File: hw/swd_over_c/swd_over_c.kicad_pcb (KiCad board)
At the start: 4 copper layers, 18.3 x 16 mm, 17 parts, among them J1 USB_C_Receptacle_USB2.0, J2 Conn_ARM_JTAG_SWD_10, P1 USB_C_Plug, U1 ATtiny24-20M

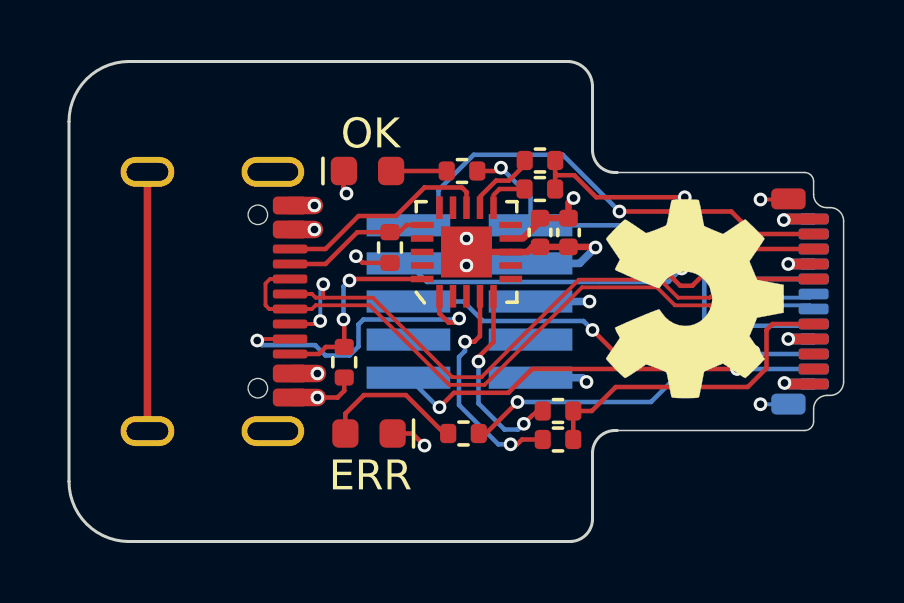
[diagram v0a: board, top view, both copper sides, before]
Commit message: SWD over USB-C v1.4!!!
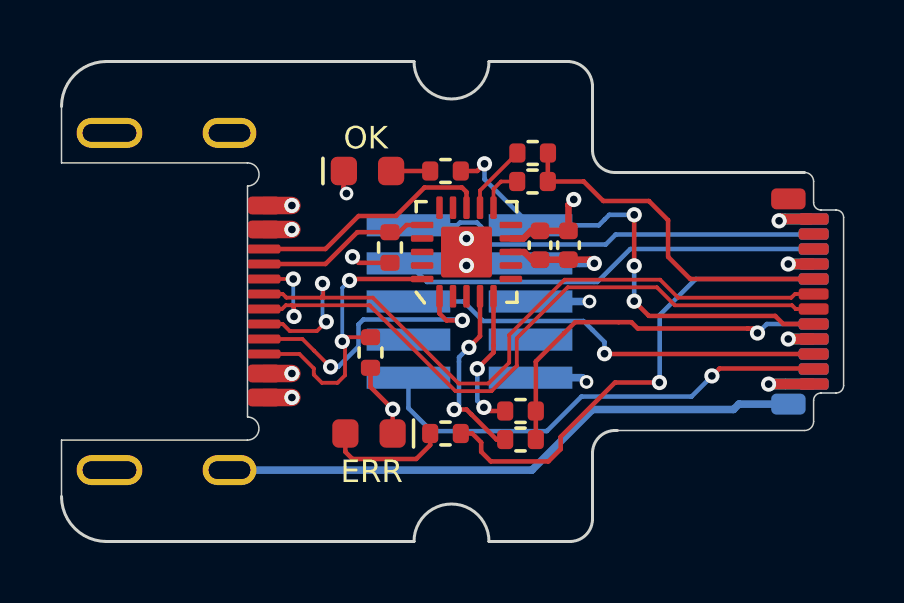
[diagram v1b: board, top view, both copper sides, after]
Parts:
- J1: value USB_C_Receptacle_USB2.0 -> USB-C Receptacle; footprint alvarop:USB4105-GF-A -> alvarop:USB4500-03
- P1: moved to F.Cu
- R3: value 10k -> 22k
- R4: value 22k -> 56k
- R5: value 22k -> 10k
- R6: value 56k -> 22k
- REF**: moved to B.Cu
- U1: footprint ultralibrarian:ATTINY24A-MMH -> ultralibrarian:ATTINY24A-MMH_MOD
- moved J1 1.42 mm to (161.2, 67.5)
- moved R5 1.25 mm to (170.3, 72.1)
- moved R6 1.25 mm to (170.3, 71.2), turned to 0 degrees
- moved R1 0.93 mm to (165.3, 69.2)
- moved R8 0.60 mm to (167.8, 71.9)
- moved R7 0.55 mm to (167.8, 63.1)
- moved C1 0.42 mm to (170.9, 65.6)
- moved C2 0.42 mm to (171.9, 65.6)
- moved R3 0.35 mm to (170.7, 63.5), turned to 180 degrees
- moved R4 0.35 mm to (170.7, 62.5), turned to 180 degrees
- moved REF** 0.15 mm to (176.1, 67.5), turned to 90 degrees
- turned P1 to -90 degrees
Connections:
- R3 pad 1: /CC1_R1 -> /CC1
- R3 pad 2: /CC1 -> /CC1_R1
- R4 pad 1: /CC1_R2 -> /CC1
- R4 pad 2: /CC1 -> /CC1_R2
- R6 pad 1: /CC2 -> /CC2_R2
- R6 pad 2: /CC2_R2 -> /CC2
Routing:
- net /SHIELD: track 57.0 -> 19.5 mm, vias 2 -> 0
- net /CC2_IN_MISO: track 6.65 -> 10.1 mm
- net /D+: track 23.2 -> 26.0 mm, vias 3 -> 2
- net /SBU2: track 14.4 -> 16.4 mm, vias 2 -> 1
- net /CC2: track 10.9 -> 12.7 mm, vias 0 -> 1
- net /CC2_R2: track 6.54 -> 4.78 mm
- net /D-: track 22.9 -> 24.5 mm, vias 1 -> 2
- net /NRST: track 14.4 -> 15.7 mm, vias 2 -> 1
- net /CC2_R1: track 7.49 -> 6.25 mm
- net VBUS: track 7.30 -> 8.39 mm
- net /SWDIO: track 15.3 -> 14.3 mm, vias 1 -> 0
- net /SCK: track 10.4 -> 9.52 mm
- net /CC1_IN_MOSI: track 4.94 -> 5.81 mm
- net /MCURST: track 7.31 -> 8.18 mm
- net /SBU1: track 15.5 -> 16.3 mm, vias 3 -> 4
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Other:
- board size 18.3 x 16 mm -> 18.5 x 16 mm
- board text added: "Leave room for USB-C plug here!"
- board text added: "v1.4"
- board text removed: "v1.3"
